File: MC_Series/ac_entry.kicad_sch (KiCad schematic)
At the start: 20 parts, among them U4 R-78E3.3-1.0

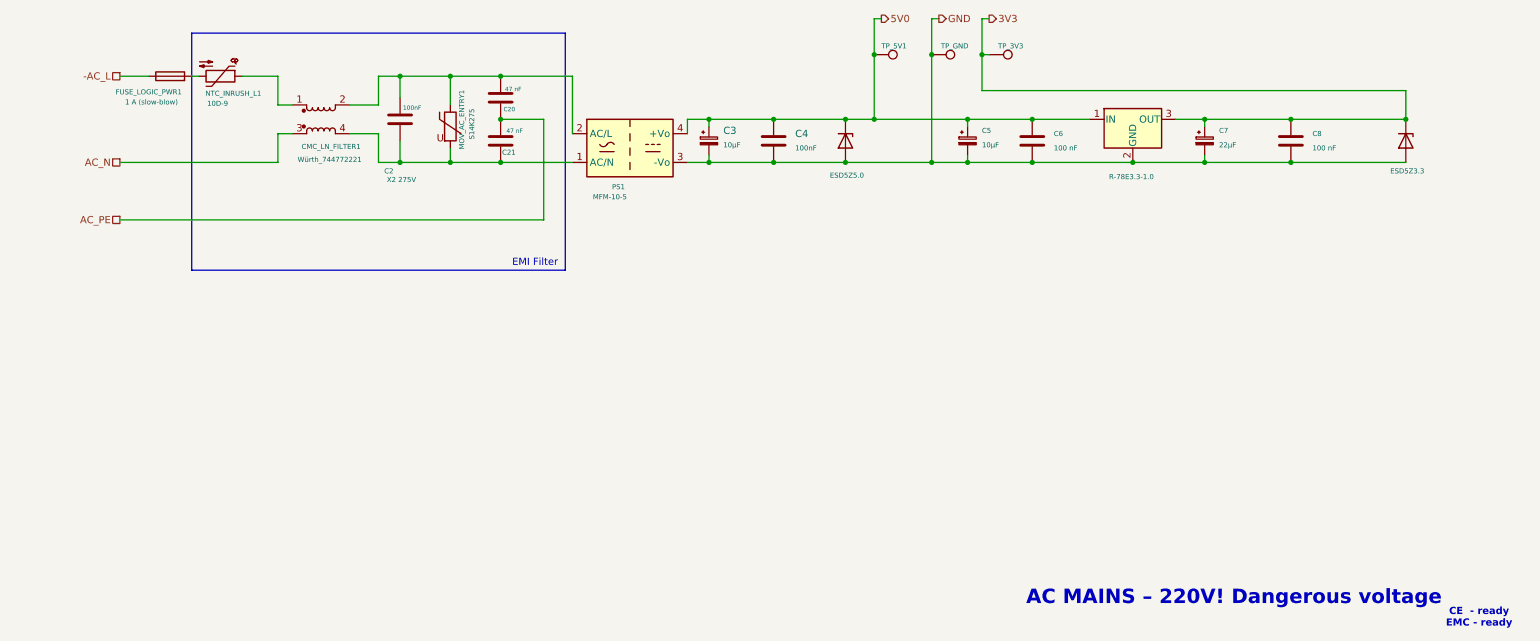
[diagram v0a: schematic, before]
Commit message: Updated MC_Series template
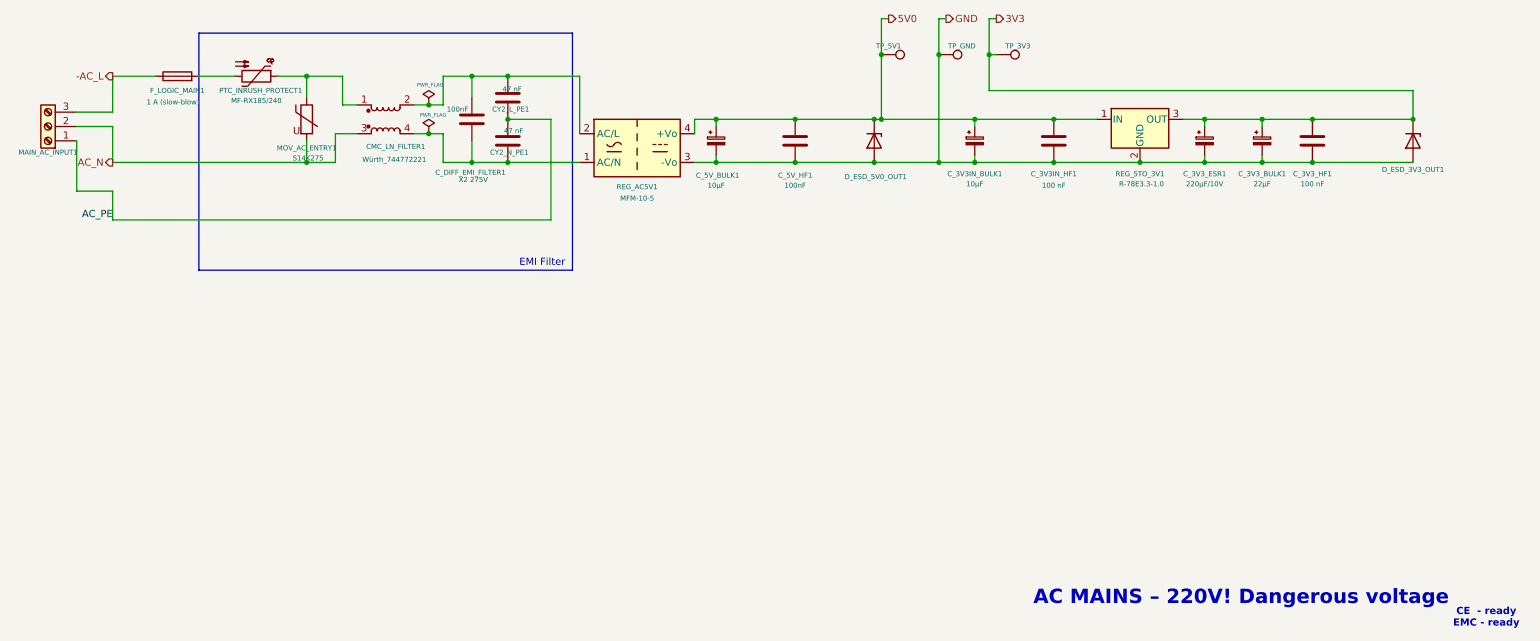
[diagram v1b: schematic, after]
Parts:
- removed NTC_INRUSH_L1: 10D-9, symbol Device:Thermistor_NTC
- added C_3V3_ESR1: 220µF/10V, symbol Device:C_Polarized_Small
- added MAIN_AC_INPUT1: Screw_Terminal_01x03, symbol Connector:Screw_Terminal_01x03
- added PTC_INRUSH_PROTECT1: MF-RX185/240, symbol Device:Thermistor_PTC
- D_ESD_5V0_OUT1: renamed from D14; value ESD5Z5.0 -> D_ESD_5V0_OUT
- renumbered C20 to CY2_L_PE1, C21 to CY2_N_PE1, C5 to C_3V3IN_BULK1, C6 to C_3V3IN_HF1, C7 to C_3V3_BULK1, C8 to C_3V3_HF1, C3 to C_5V_BULK1, C4 to C_5V_HF1, C2 to C_DIFF_EMI_FILTER1, D13 to D_ESD_3V3_OUT1, FUSE_LOGIC_PWR1 to F_LOGIC_MAIN1, U4 to REG_5TO_3V1, PS1 to REG_AC5V1
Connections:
- net 3V3: now also C_3V3_ESR1.1
- net AC_N: now also MOV_AC_ENTRY1.2, MAIN_AC_INPUT1.2 (Pin_2)
- net AC_PE: now also MAIN_AC_INPUT1.1 (Pin_1)
- net GND: now also C_3V3_ESR1.2
- net ­AC_L: now also MAIN_AC_INPUT1.3 (Pin_3)
- net at F_LOGIC_MAIN1.2: now also PTC_INRUSH_PROTECT1.2
- net at CMC_LN_FILTER1.1: now also MOV_AC_ENTRY1.1, PTC_INRUSH_PROTECT1.1
- net at CMC_LN_FILTER1.2, CY2_L_PE1.1, C_DIFF_EMI_FILTER1.1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: no longer MOV_AC_ENTRY1.1
- net at CMC_LN_FILTER1.4, CY2_N_PE1.2, C_DIFF_EMI_FILTER1.2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: no longer MOV_AC_ENTRY1.2
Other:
- moved on the sheet: CMC_LN_FILTER1, CY2_L_PE1, CY2_N_PE1, C_3V3IN_BULK1, C_3V3IN_HF1, C_3V3_BULK1, C_3V3_HF1, C_5V_BULK1, C_5V_HF1, C_DIFF_EMI_FILTER1, F_LOGIC_MAIN1, MOV_AC_ENTRY1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
